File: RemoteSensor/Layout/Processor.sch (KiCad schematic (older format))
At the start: 21 parts, among them J3 LCD_HEADER, J4 PRG_HEADER, Q3 2N7002, U7 ESP-12F, U8 LM50CIM3, U9 MCP23008-E_P

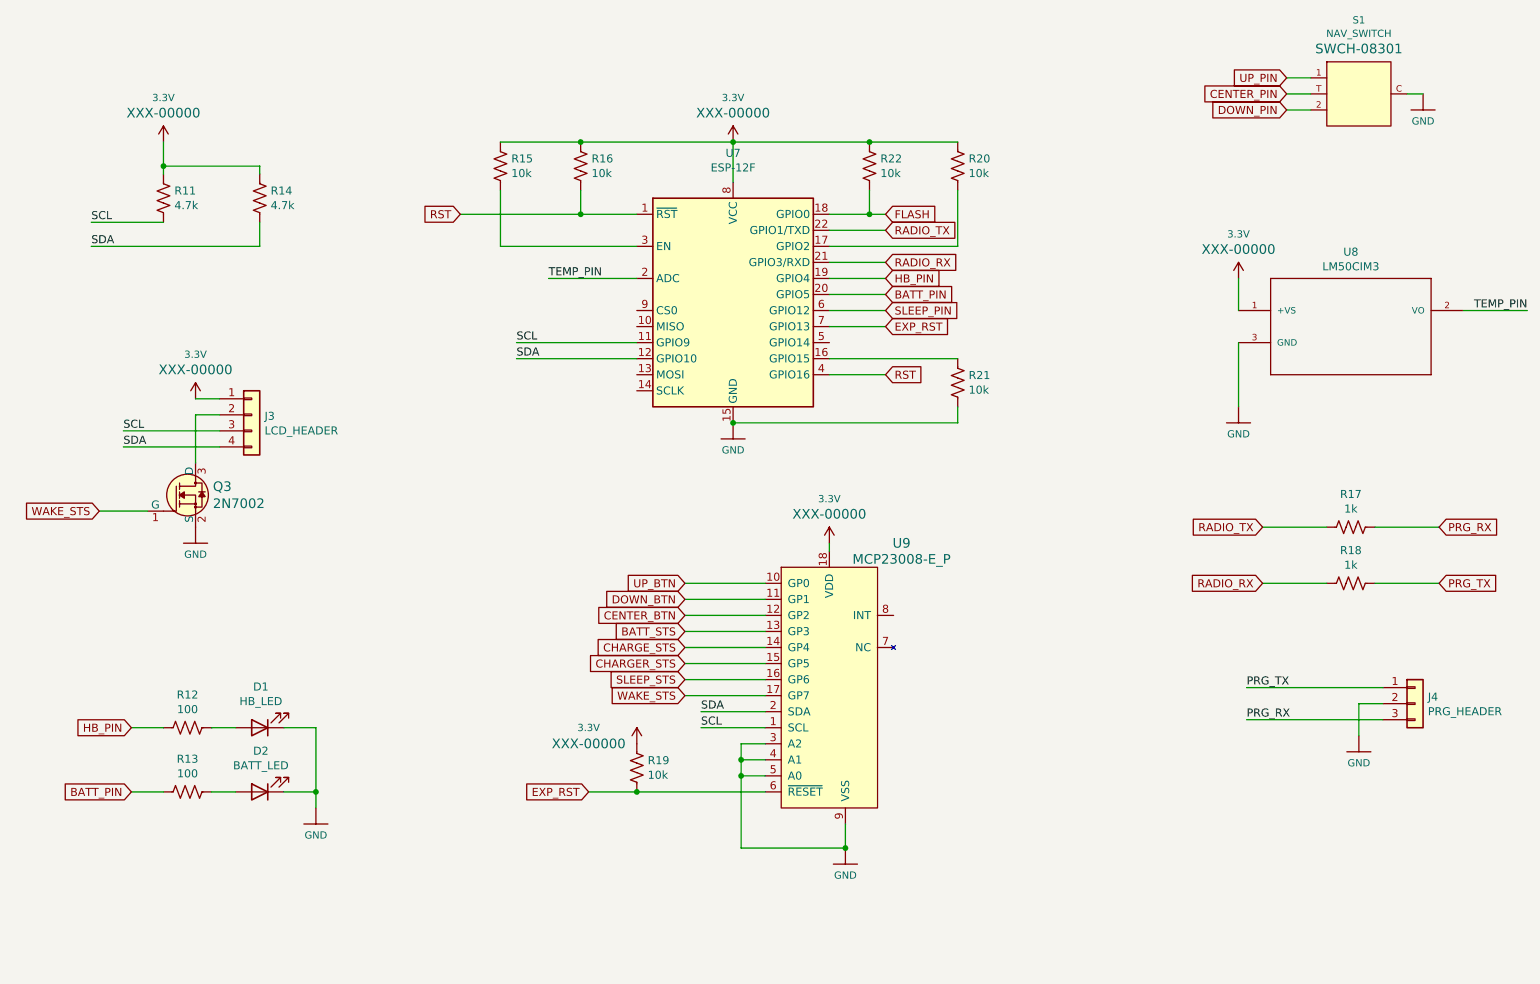
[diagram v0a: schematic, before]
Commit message: Edit layout
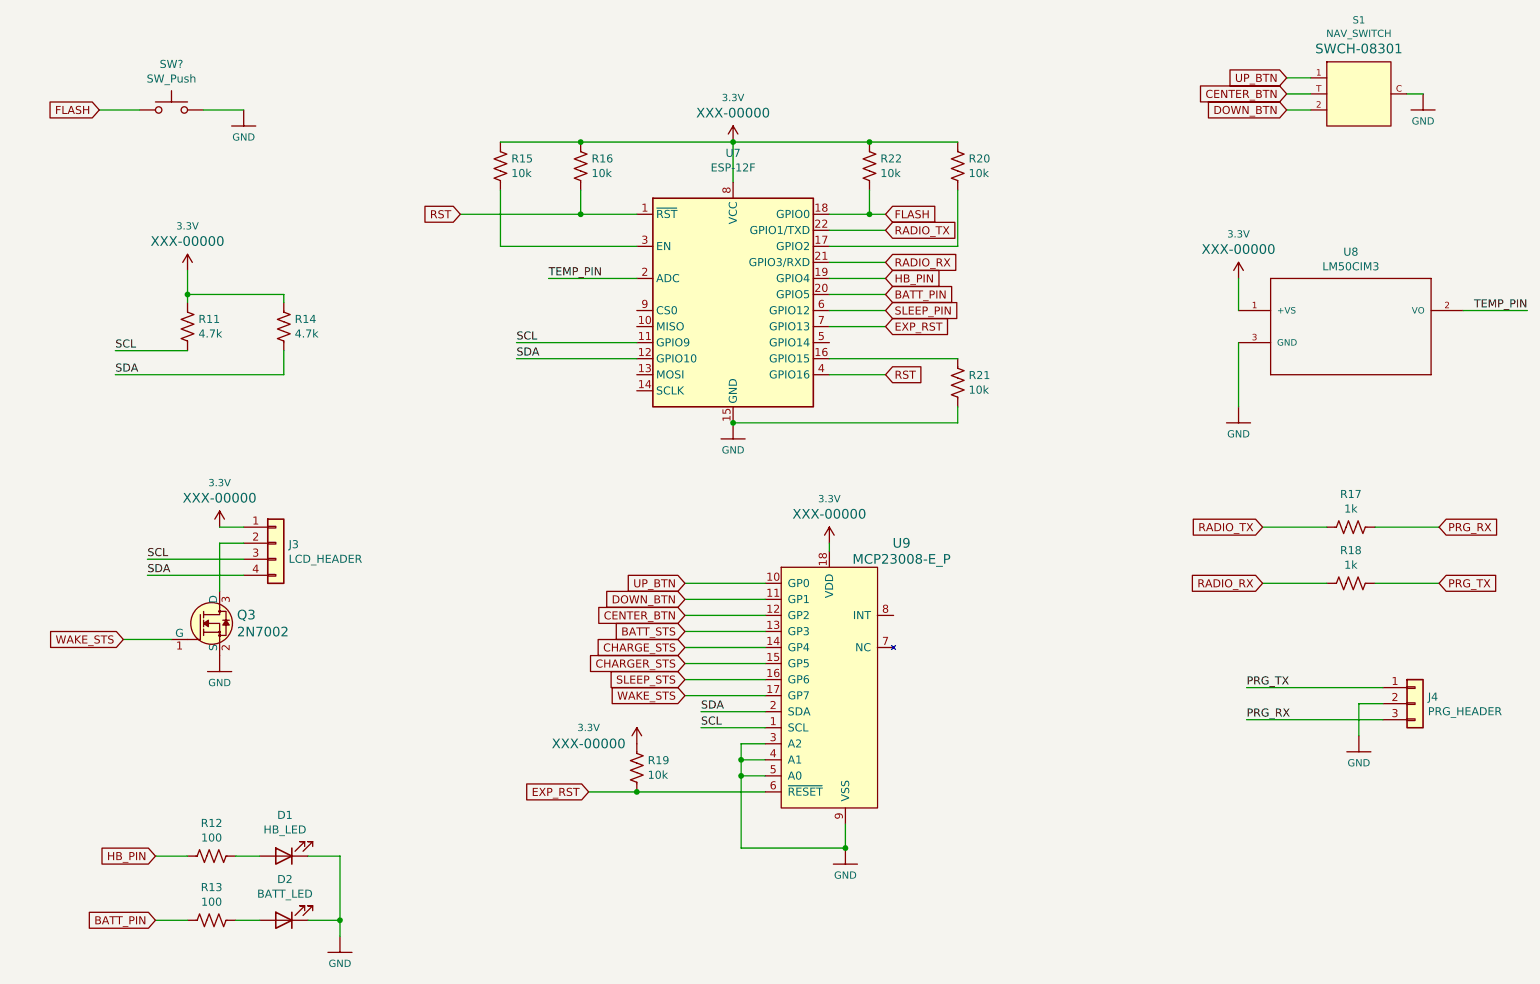
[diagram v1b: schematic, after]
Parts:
- added SW?: SW_Push, Button_Switch_SMD:SW_SPST_TL3342, symbol Switch:SW_Push
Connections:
- net CENTER_PIN is gone; now on net CENTER_BTN: S1.T
- net DOWN_PIN is gone; now on net DOWN_BTN: S1.2
- net UP_PIN is gone; now on net UP_BTN: S1.1
- net FLASH: now also SW?.1
- net GND: now also SW?.2
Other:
- moved on the sheet: D1, D2, J3, Q3, R11, R12, R13, R14
